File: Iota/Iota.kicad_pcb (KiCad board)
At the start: 2 copper layers, 28.7 x 42.3 mm, 21 parts, among them J1 USB_B_Mini, J2 Conn_01x12_Male, J3 Conn_01x12_Male, J4 Conn_01x05_Male, SW1 SW_DIP_x01, U1 ATmega32U4-AU, Y1 16MHz

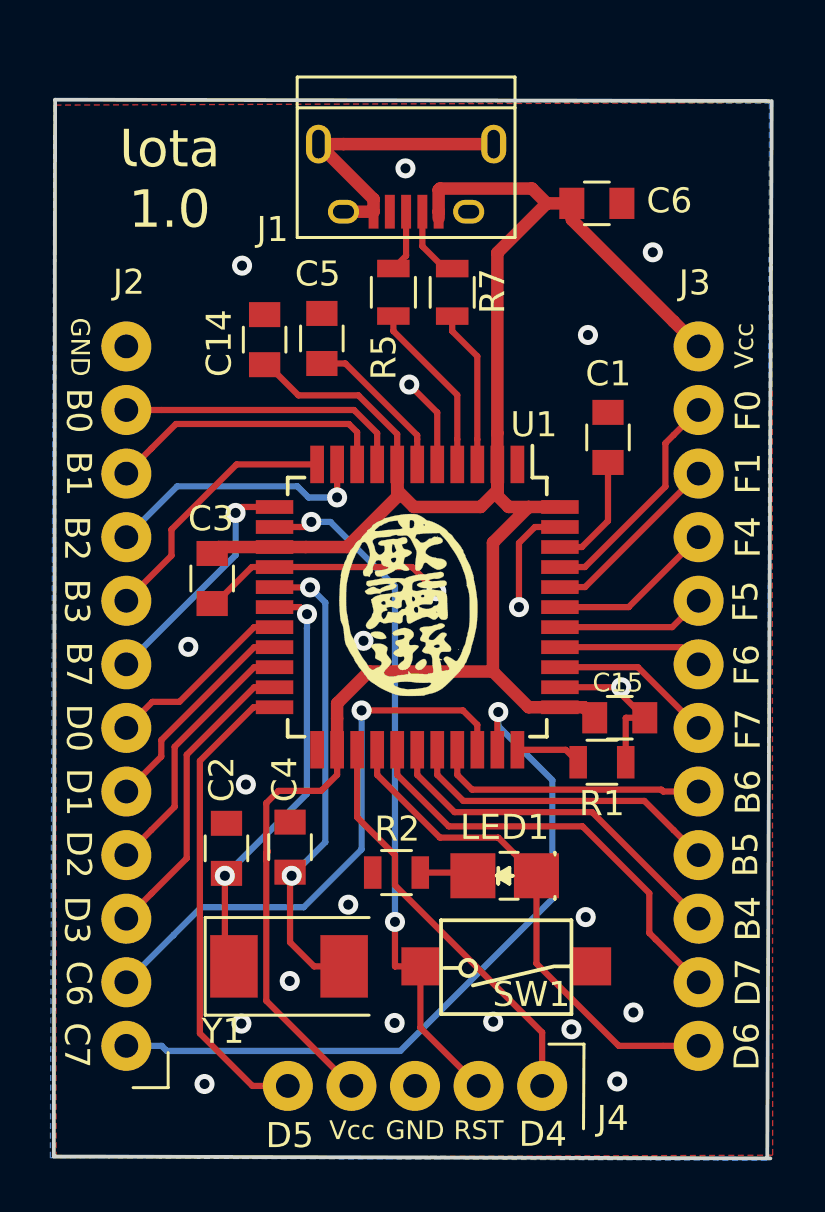
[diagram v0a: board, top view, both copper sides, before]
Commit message: Minor changes
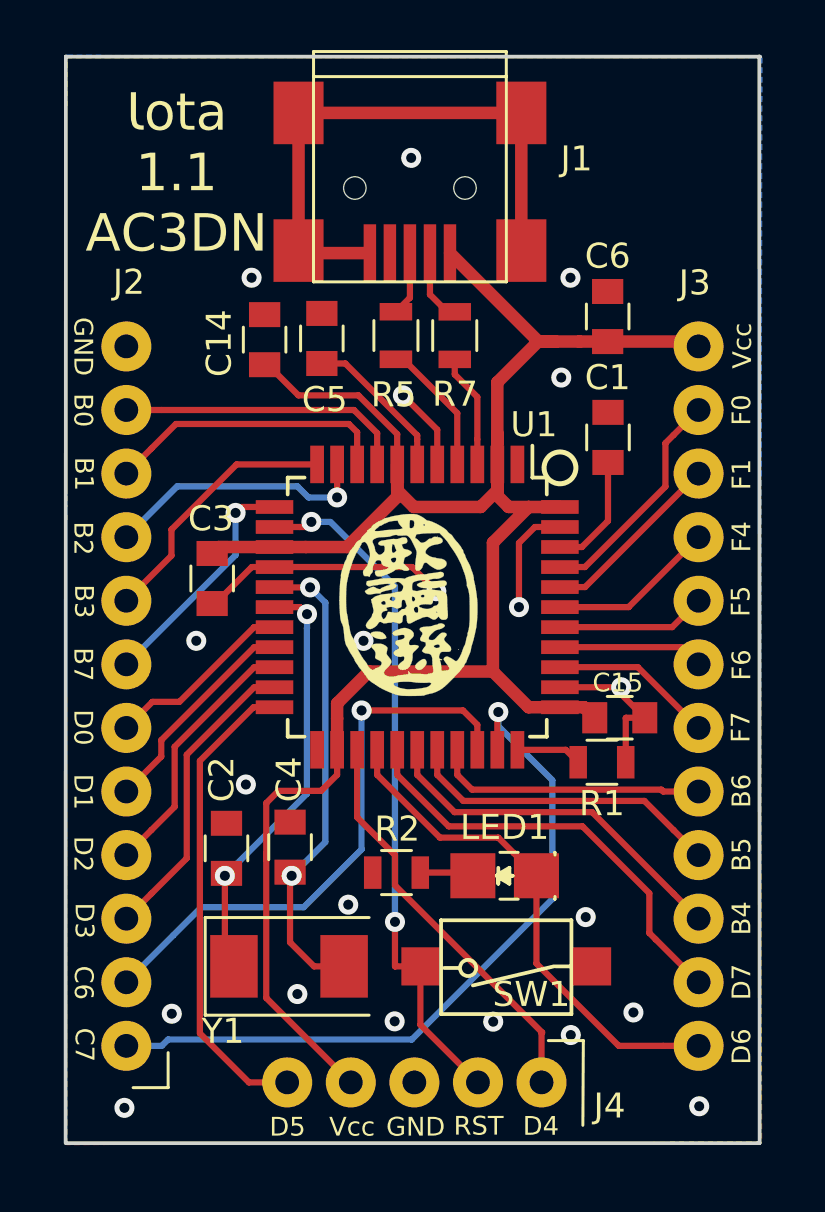
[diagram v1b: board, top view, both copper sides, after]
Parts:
- J1: footprint Connectors:USB_Micro-B -> Connectors:USB_Mini-B
- moved C6 4.54 mm to (141.4, 70.2), turned to 270 degrees
- moved R7 1.73 mm to (135.3, 70.9)
- moved R5 1.73 mm to (132.9, 70.9)
- moved J1 0.25 mm to (133.5, 64.8), turned to 270 degrees
- moved J4 0.14 mm to (138.8, 100.8)
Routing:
- net GND: track 36.7 -> 47.3 mm
- net Vcc: track 92.1 -> 83.7 mm
- net D-: track 6.34 -> 4.57 mm
- net D+: track 6.98 -> 5.39 mm
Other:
- board size 28.7 x 42.3 mm -> 27.7 x 43.4 mm
- board text added: "Ɩota 1.1 AC3DN"
- board text removed: "Ɩota 1.0"
